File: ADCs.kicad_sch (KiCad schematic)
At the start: 22 parts, among them J10 Conn_01x03, J11 Conn_01x03, J12 Conn_01x03, J13 Conn_01x03, J14 Conn_01x03, J15 Conn_01x03, J16 Conn_01x03, J17 Conn_01x03, J2 Conn_01x03, J3 Conn_01x03, J4 Conn_01x03, J5 Conn_01x03, J6 Conn_01x03, J7 Conn_01x03, J8 Conn_01x03, J9 Conn_01x03, U3 ADS7828, U4 ADS7828

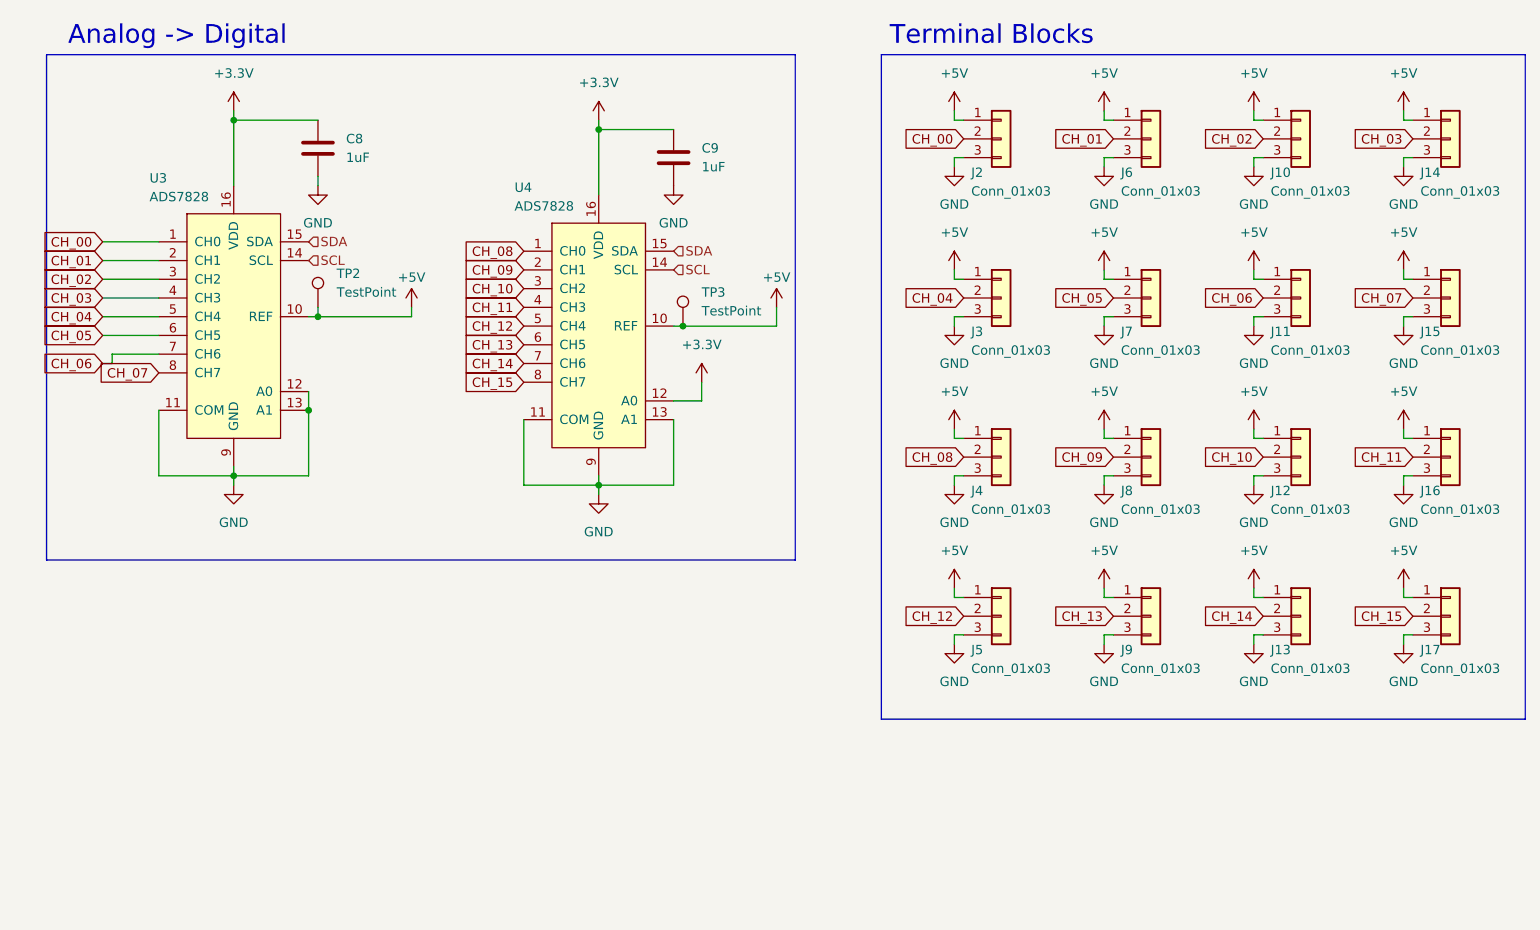
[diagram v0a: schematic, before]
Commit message: lots🅿️
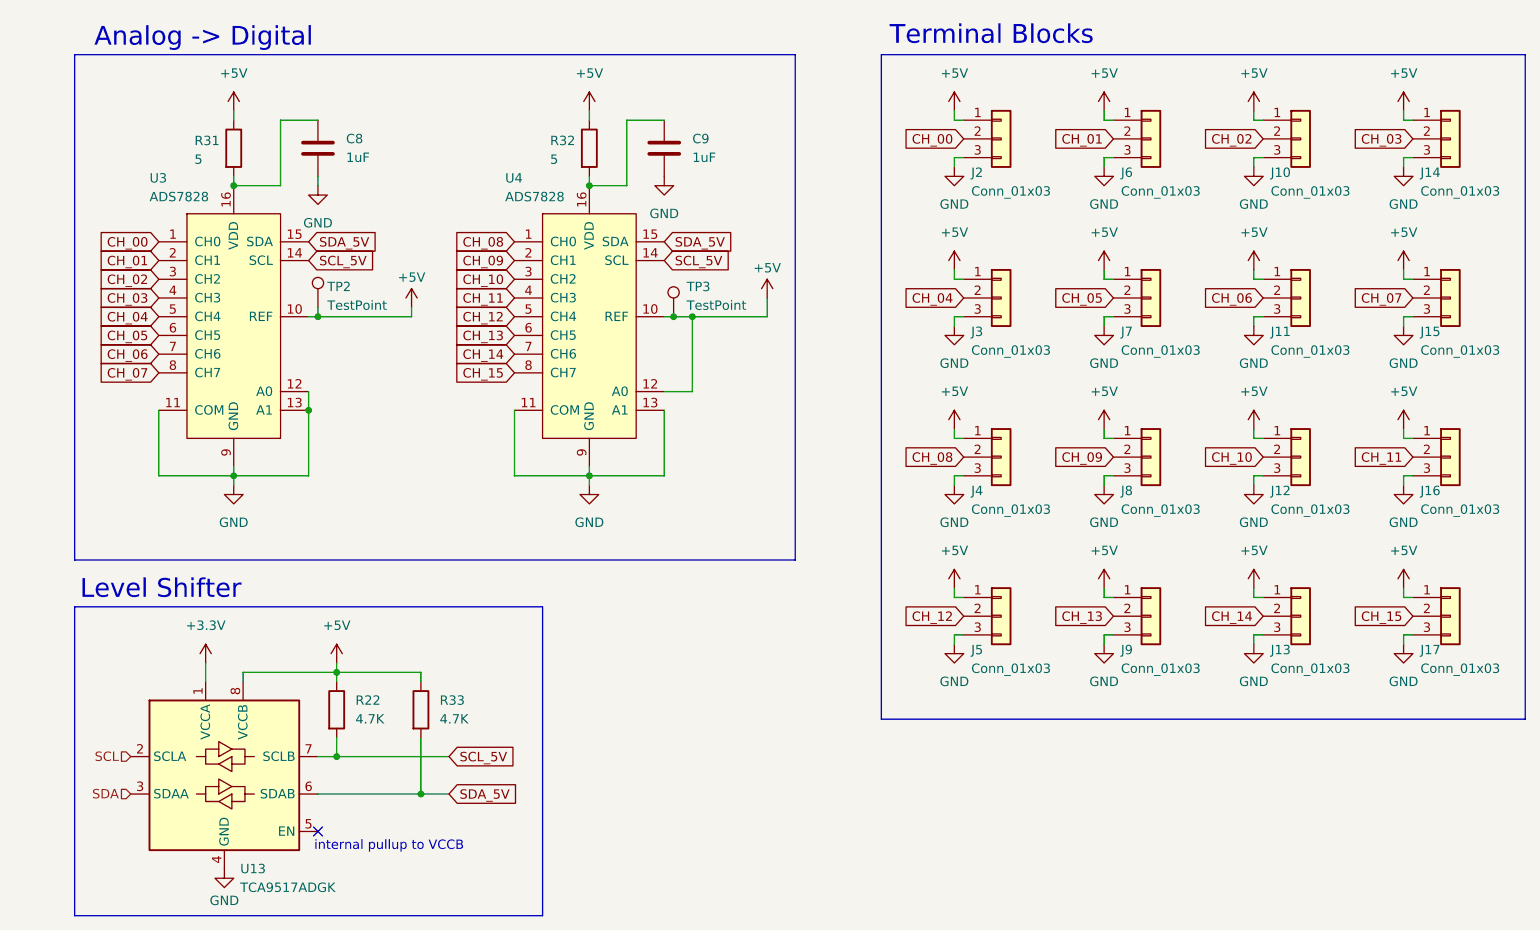
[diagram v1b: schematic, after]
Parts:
- added R22, R33: 4.7K, Resistor_SMD:R_0402_1005Metric, symbol Device:R
- added R31, R32: 5, symbol Device:R
- added U13: TCA9517ADGK, Package_SO:VSSOP-8_3x3mm_P0.65mm, symbol Logic_LevelTranslator:TCA9517ADGK
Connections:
- net +3.3V: now also U13.1 (VCCA); no longer C8.1, C9.1, U3.16 (VDD), U4.12 (A0), U4.16 (VDD)
- net +5V: now also U4.12 (A0), R22.1, R31.1, R32.1, R33.1, U13.8 (VCCB)
- net GND: now also U13.4 (GND)
- net SCL: now also U13.2 (SCLA); no longer U3.14 (SCL), U4.14 (SCL)
- net SDA: now also U13.3 (SDAA); no longer U3.15 (SDA), U4.15 (SDA)
- new net: C9.1, R32.2, U4.16 (VDD)
- new net: C8.1, R31.2, U3.16 (VDD)
- new net SCL_5V: R22.2, U13.7 (SCLB), U3.14 (SCL), U4.14 (SCL)
- new net SDA_5V: R33.2, U13.6 (SDAB), U3.15 (SDA), U4.15 (SDA)
- no-connect marks 0 -> 1
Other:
- note added: "Level Shifter"
- note added: "internal pullup to VCCB"
- moved on the sheet: C9, TP3, U4
